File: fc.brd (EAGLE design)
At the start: 160 x 100 mm, 64 parts, among them IC1 FT230XQ, IC2 BN055, U2 ATMEGA2560-16AU100A-M, Y1 16MHz, Y2 32.768kHz

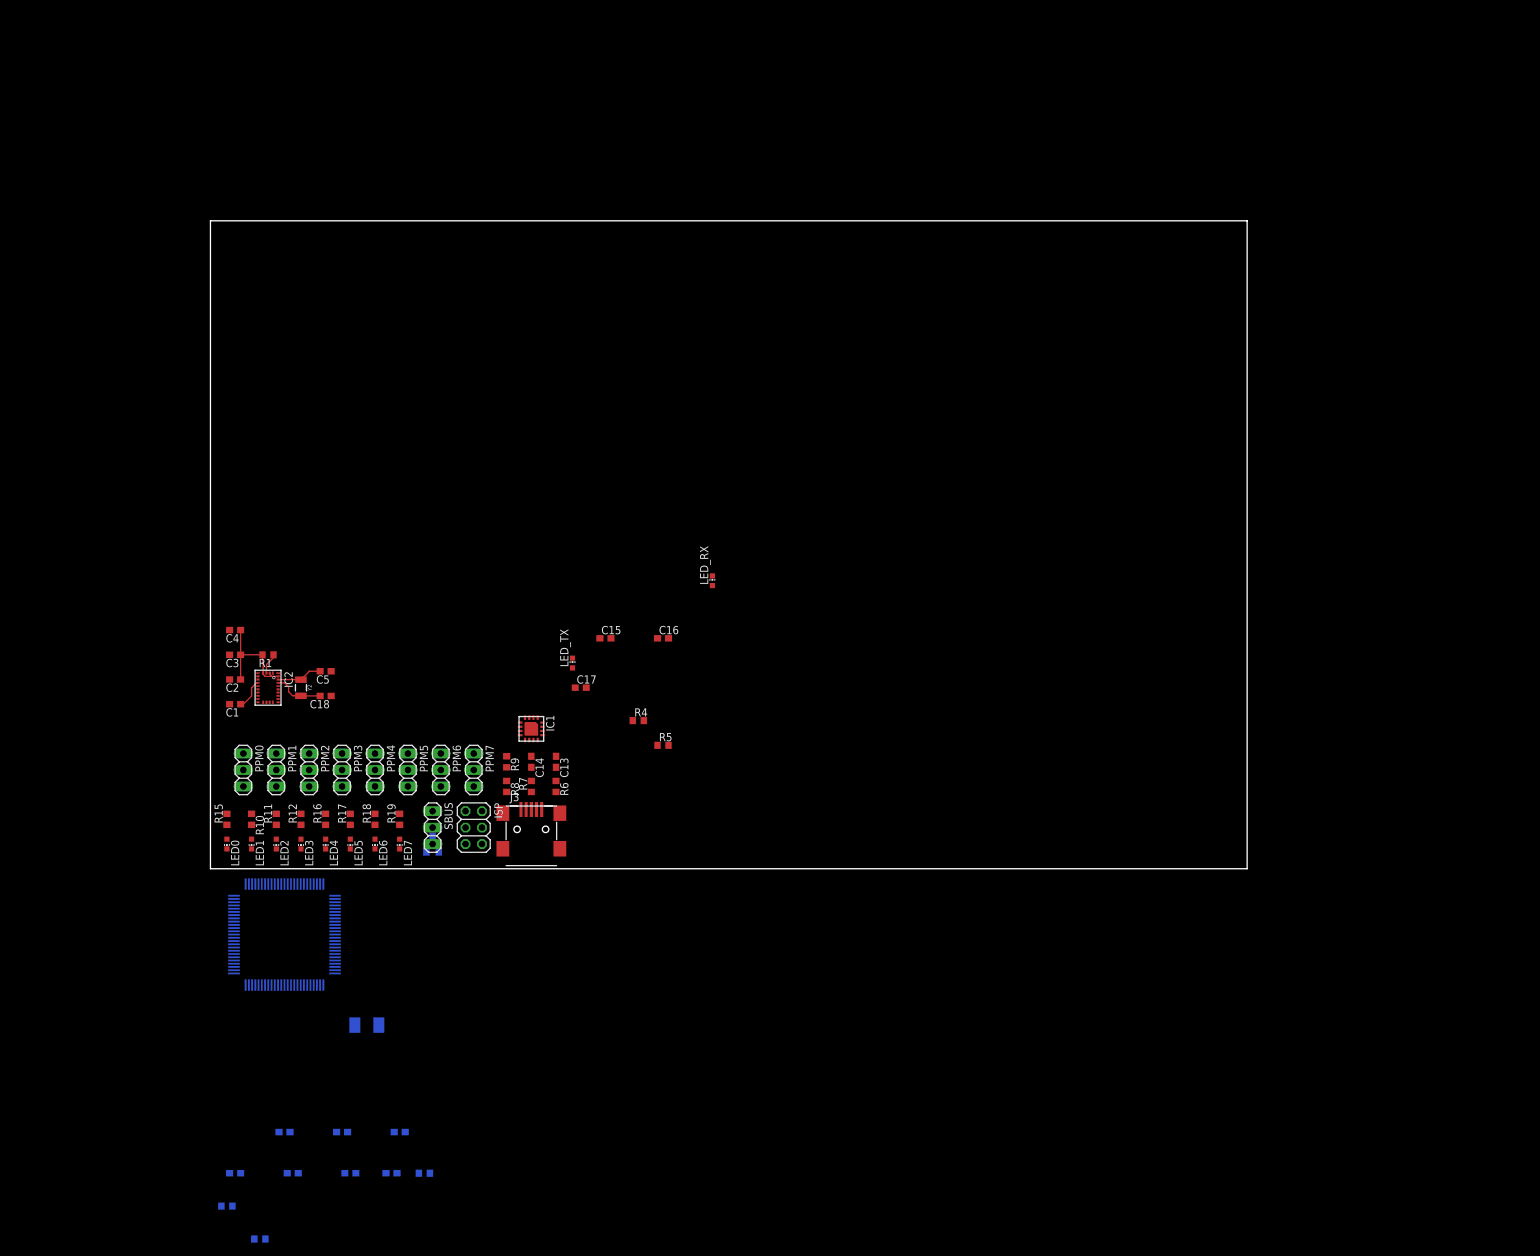
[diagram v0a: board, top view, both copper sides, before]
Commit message: Initial draft for the layout
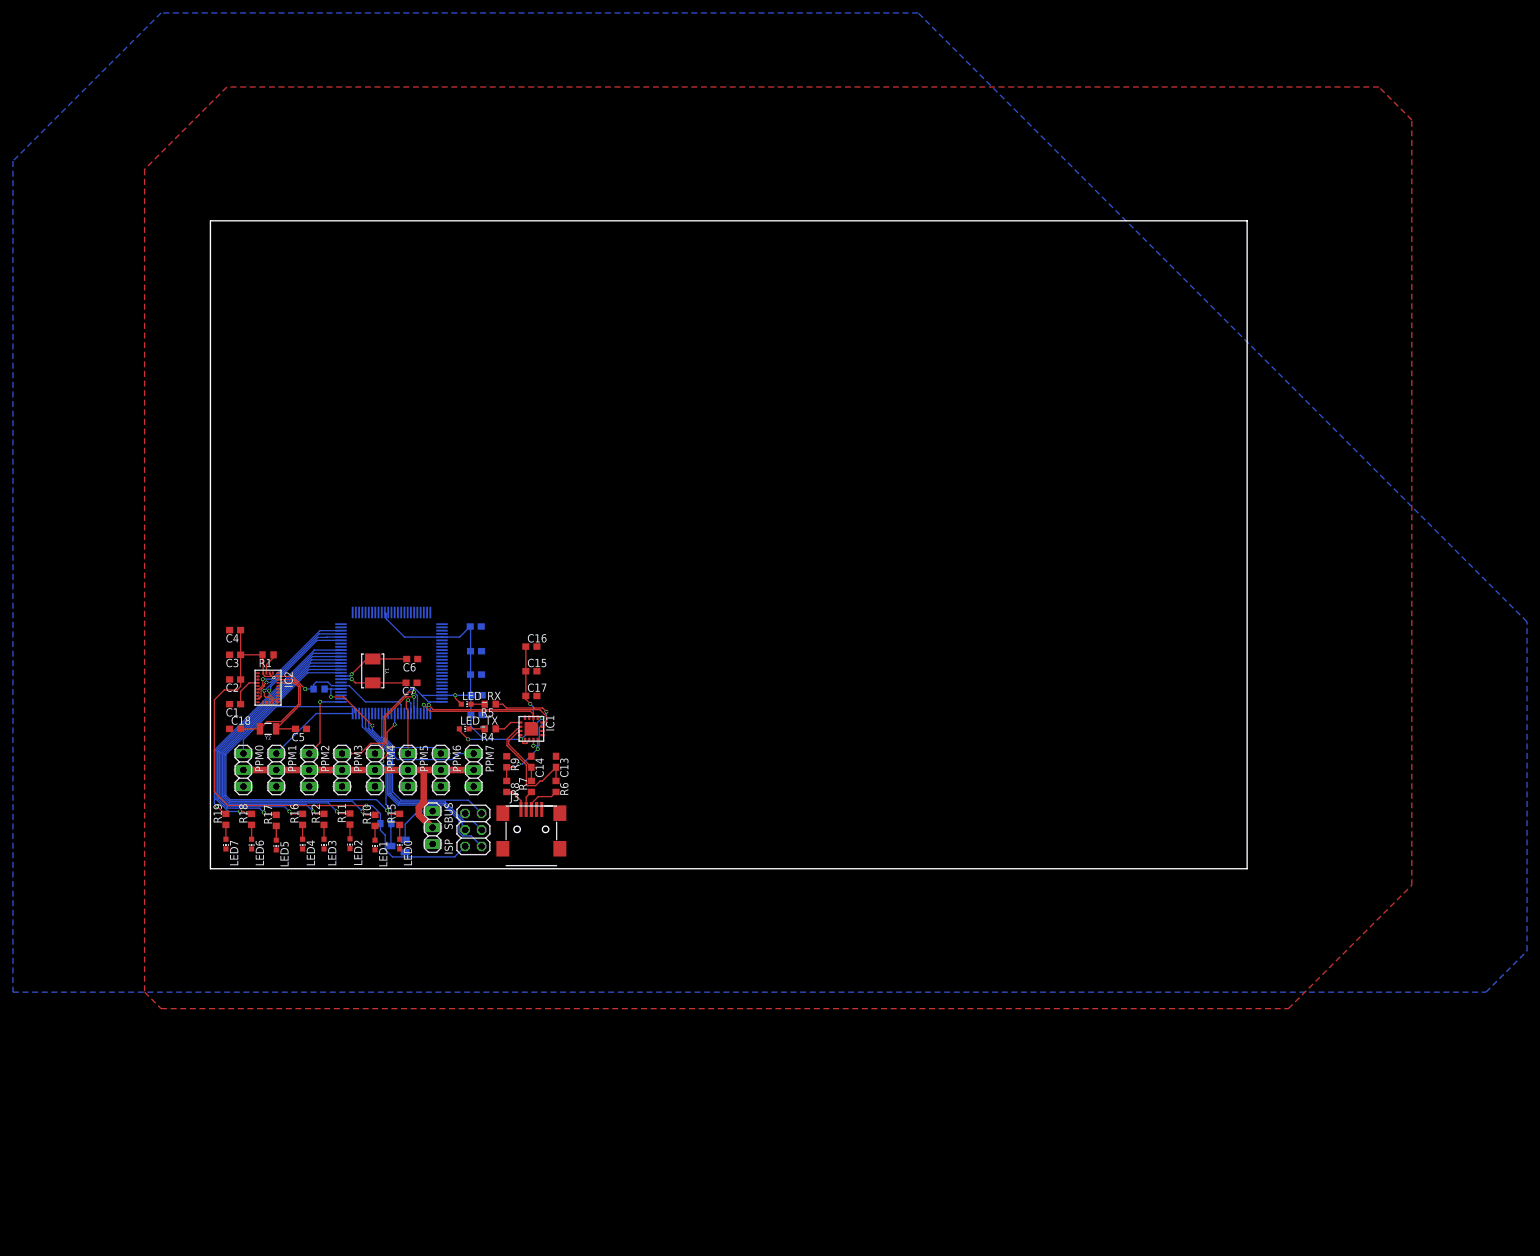
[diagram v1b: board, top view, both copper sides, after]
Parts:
- removed R13, R14: 10k, rcl:R0603
- moved C12 89.0 mm to (40.9, 37.4), turned to 180 degrees
- moved C11 88.7 mm to (41.0, 33.6), turned to 180 degrees
- moved R3 85.4 mm to (16.8, 27.7)
- moved C6 79.9 mm to (31.1, 32.4), flipped to the top, turned to 180 degrees
- moved C8 76.6 mm to (41.0, 30.0), turned to 180 degrees
- moved C7 75.8 mm to (31.0, 28.7), flipped to the top, turned to 180 degrees
- moved C9 70.5 mm to (41.1, 26.8), turned to 180 degrees
- moved C10 65.4 mm to (41.0, 23.7), turned to 180 degrees
- moved Y1 54.7 mm to (25.0, 30.5), flipped to the top, turned to 270 degrees
- moved U2 45.0 mm to (27.9, 31.8), turned to 90 degrees
- moved LED_RX 42.5 mm to (39.5, 25.4), turned to 270 degrees
- moved R5 27.4 mm to (43.2, 25.4), turned to 180 degrees
- moved LED7 26.8 mm to (2.39, 3.81)
- moved R19 26.8 mm to (2.39, 7.62)
- moved LED0 26.7 mm to (29.2, 3.81)
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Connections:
- removed net SCL: R13.1, U2.43
- removed net SDA: R14.1, U2.44
- net +3V3: now also C10.1, C11.1, C12.1, C15.1, C16.1, C17.1, C8.1, C9.1, IC1.1, IC1.10, IC1.8, ISP.2, LED_RX.A, LED_TX.A, R3.2, U2.10, U2.100, U2.31, U2.61, U2.80, U2.98; no longer R13.2, R14.2
- net +5V: no longer C10.1, C11.1, C12.1, C15.1, C16.1, C17.1, C8.1, C9.1, IC1.1, IC1.10, IC1.8, ISP.2, LED_RX.A, LED_TX.A, R3.2, U2.10, U2.100, U2.31, U2.61, U2.80, U2.98
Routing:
- net +3V3: track 17.1 -> 191.2 mm, vias 0 -> 7
- net +5V: track 0.00 -> 71.1 mm
- net LED0: track 0.00 -> 57.3 mm, vias 0 -> 1
- net LED1: track 0.00 -> 54.4 mm, vias 0 -> 1
- net LED2: track 0.00 -> 51.3 mm, vias 0 -> 1
- net LED3: track 0.00 -> 48.1 mm, vias 0 -> 1
- net LED4: track 0.00 -> 45.6 mm, vias 0 -> 1
- net LED5: track 0.00 -> 42.5 mm, vias 0 -> 1
- net LED6: track 0.00 -> 39.4 mm, vias 0 -> 1
- net !RESET: track 0.00 -> 38.6 mm, vias 0 -> 2
- net LED7: track 0.00 -> 36.6 mm, vias 0 -> 1
- net MISO: track 0.00 -> 33.0 mm
- net SCK: track 0.00 -> 30.1 mm
- net MOSI: track 0.00 -> 28.5 mm
- net PPM0: track 0.00 -> 22.5 mm
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- added copper zone on layer 1, net GND
- added copper zone on layer 16, net GND
